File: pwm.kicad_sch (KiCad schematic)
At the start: 11 parts, among them IC1 UCC28180D, Q4 T2N7002AK, U3 UCC21520DW, U9 CD4053B

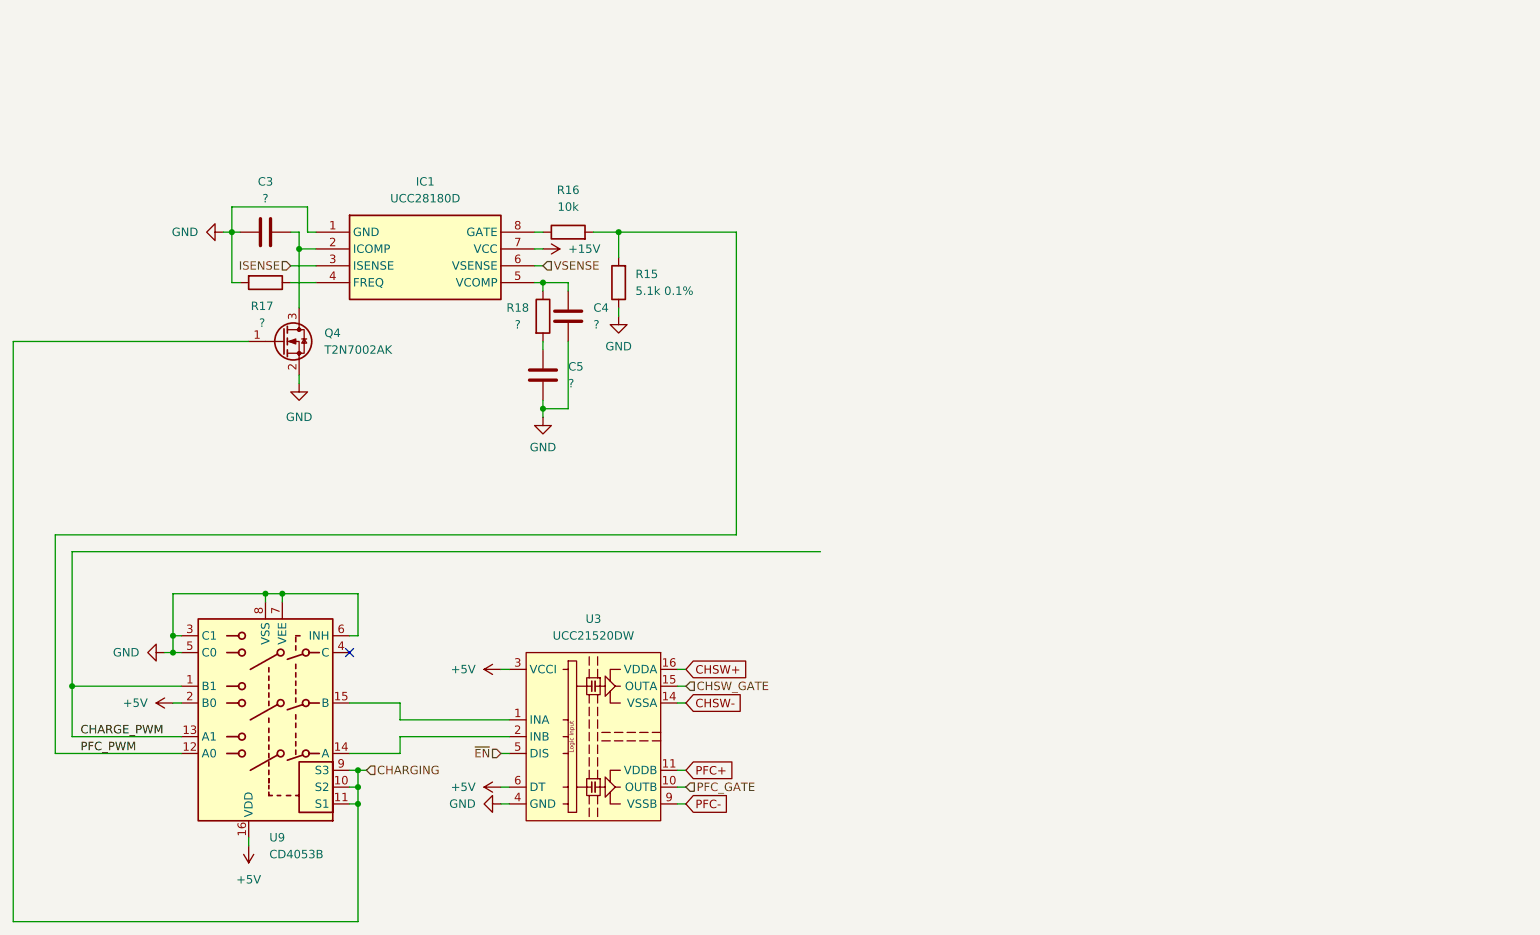
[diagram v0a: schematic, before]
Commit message: finish initial schematic
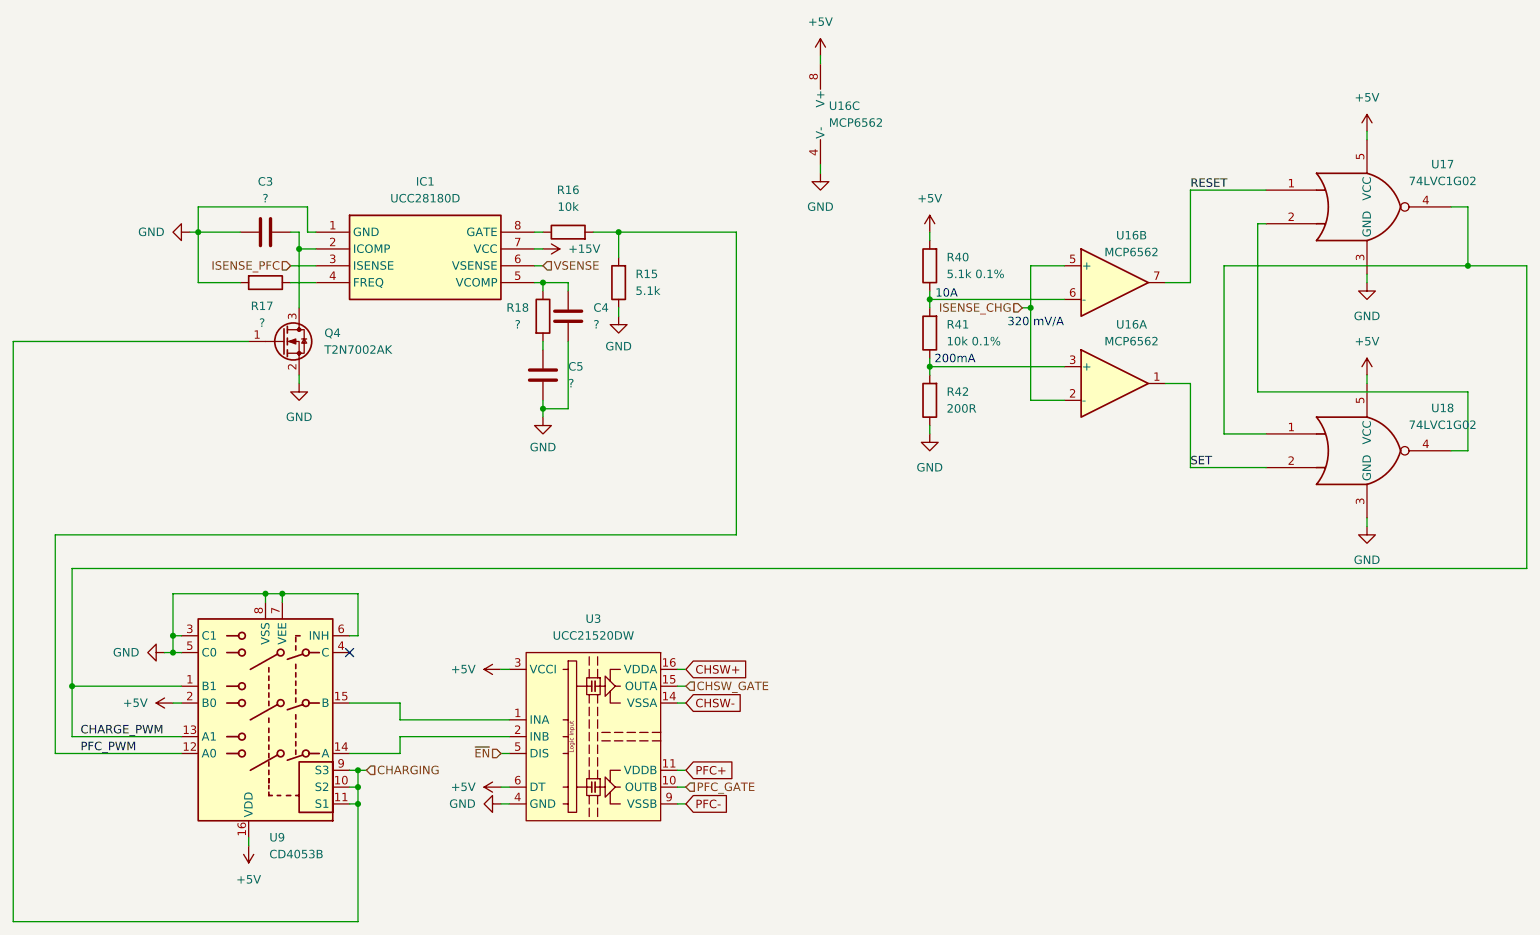
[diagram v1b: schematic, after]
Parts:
- added R40: 5.1k 0.1%, Resistor_SMD:R_0805_2012Metric, symbol Device:R
- added R41: 10k 0.1%, Resistor_SMD:R_0805_2012Metric, symbol Device:R
- added R42: 200R, Resistor_SMD:R_0805_2012Metric, symbol Device:R
- added U16: MCP6562, Package_SO:SOIC-8_3.9x4.9mm_P1.27mm, symbol Comparator:MCP6562
- added U17, U18: 74LVC1G02, Package_TO_SOT_SMD:SOT-23-5, symbol 74xGxx:74LVC1G02
- R15: value 5.1k 0.1% -> 5.1k
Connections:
- net +5V: now also R40.2, U16.8 (V+), U17.5 (VCC), U18.5 (VCC)
- net CHARGE_PWM: now also U17.4, U18.1
- net GND: now also R42.1, U16.4 (V-), U17.3 (GND), U18.3 (GND)
- net ISENSE renamed ISENSE_PFC
- new net: U17.2, U18.4
- new net: R41.1, R42.2, U16.3 (+)
- new net: R40.1, R41.2, U16.6 (-)
- new net ISENSE_CHG: U16.2 (-), U16.5 (+)
- new net RESET: U16.7, U17.1
- new net SET: U16.1, U18.2
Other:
- note added: "10A"
- note added: "200mA"
- note added: "320 mV/A"
